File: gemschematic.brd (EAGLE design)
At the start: 90.2 x 61.9 mm, 57 parts, among them J1 USB, J3 QWIIC, J5 U.FL, Q1 2N3904, Q2 BSS138, Q3 MBT3904DW1T1, U1 ESP-WROOM-32NARROW, U2 AP2112K-3.3, U3 3.3V, U4 RFM96W, U5 CH340C, U6 BMP180, U7 STM32L073RZT6, X1 GPS_PA1010D

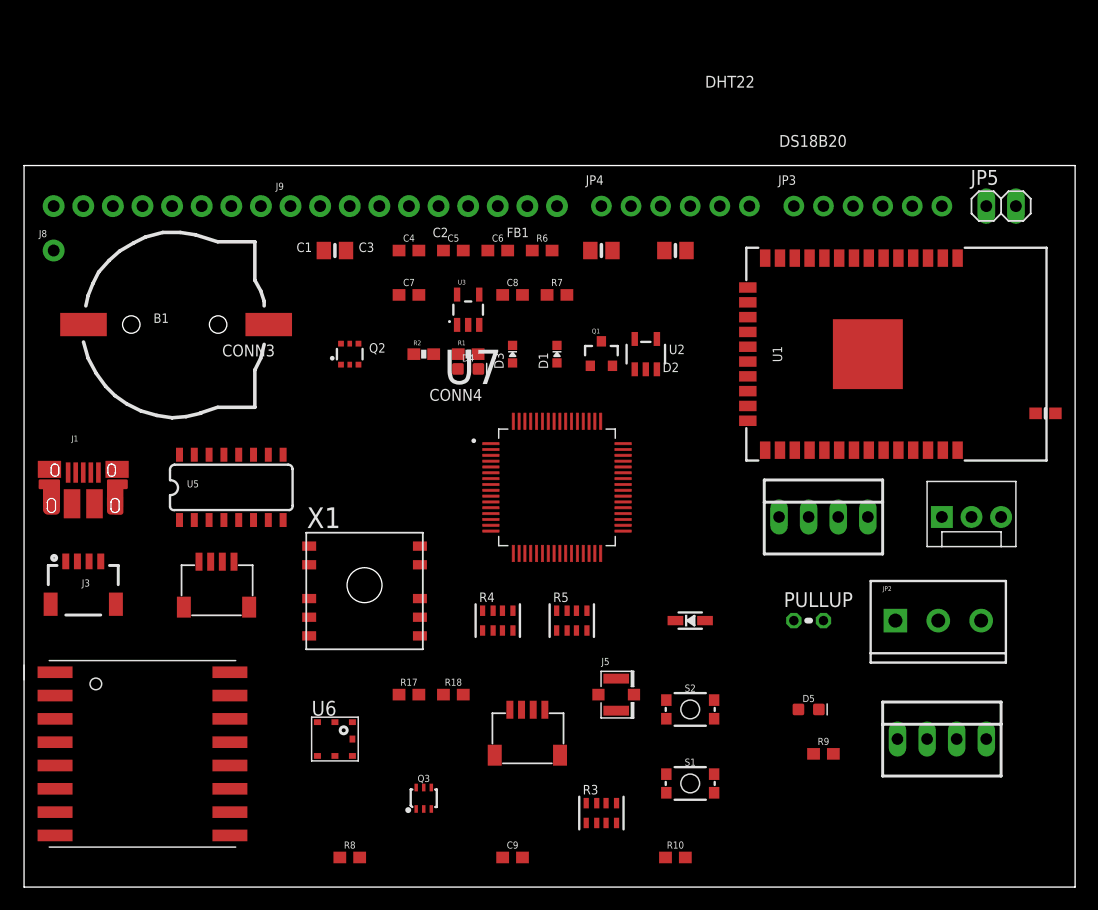
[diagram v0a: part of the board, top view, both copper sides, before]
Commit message: Add files via upload
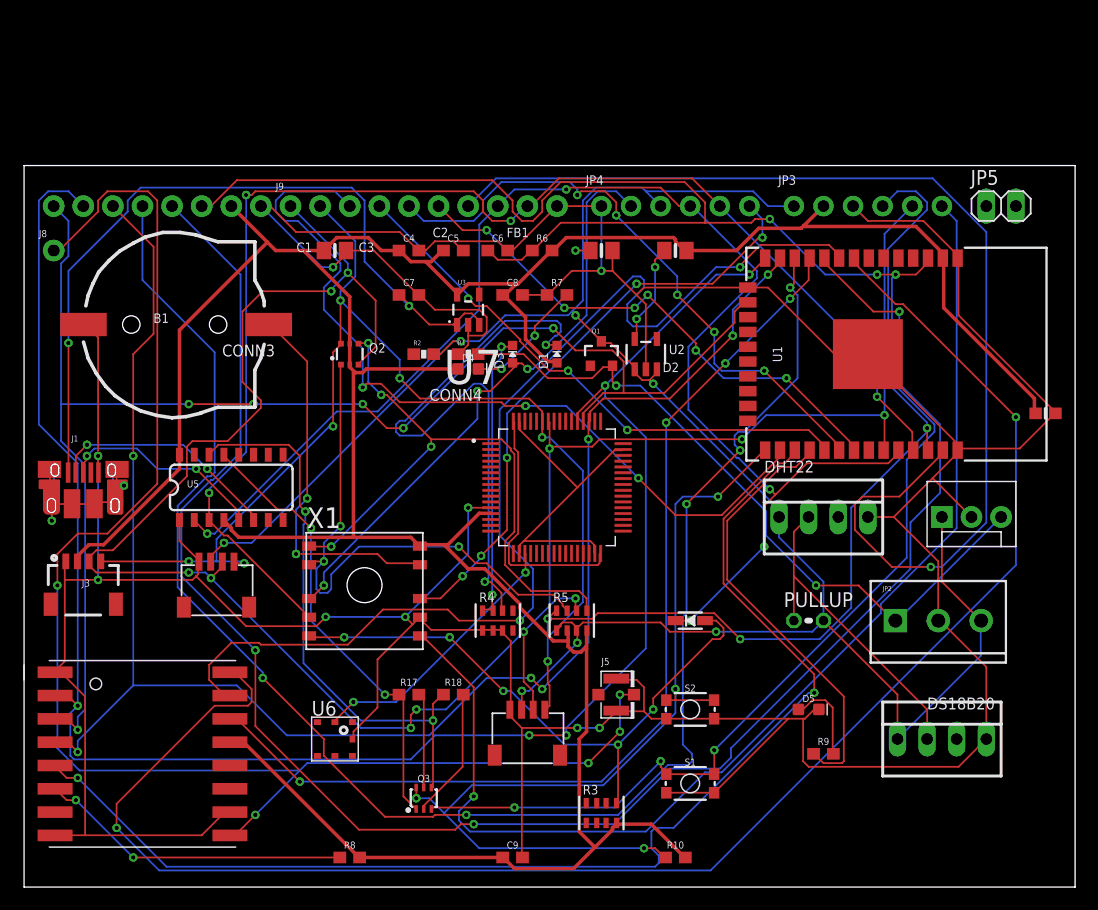
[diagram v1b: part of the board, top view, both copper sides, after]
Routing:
- net GND: track 0.00 -> 423.1 mm, vias 0 -> 9
- net 3.3V: track 0.00 -> 279.9 mm
- net SDA: track 0.00 -> 189.3 mm, vias 0 -> 11
- net VCC: track 0.00 -> 183.9 mm, vias 0 -> 8
- net SCL: track 0.00 -> 179.1 mm, vias 0 -> 10
- net RESET: track 0.00 -> 171.9 mm, vias 0 -> 6
- net MISO: track 0.00 -> 156.4 mm, vias 0 -> 5
- net IO25: track 0.00 -> 154.6 mm, vias 0 -> 3
- net RFM_DIO2/32: track 0.00 -> 142.8 mm, vias 0 -> 2
- net SCK: track 0.00 -> 141.3 mm, vias 0 -> 7
- net IO27: track 0.00 -> 140.8 mm, vias 0 -> 5
- net ANT: track 0.00 -> 127.0 mm, vias 0 -> 5
- net MOSI: track 0.00 -> 125.1 mm, vias 0 -> 6
- net RXI: track 0.00 -> 120.5 mm, vias 0 -> 5
- net TXO: track 0.00 -> 114.0 mm, vias 0 -> 4
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
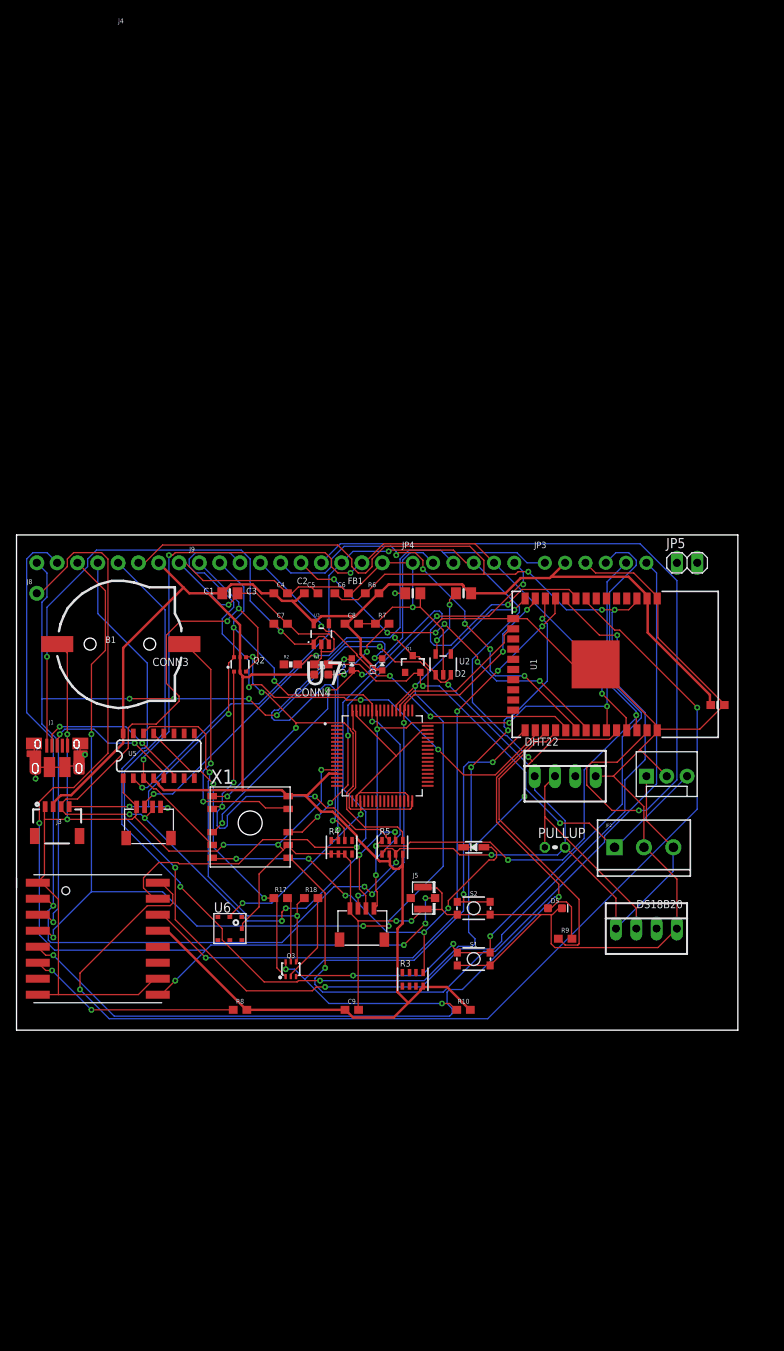
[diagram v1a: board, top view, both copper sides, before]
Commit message: Add files via upload
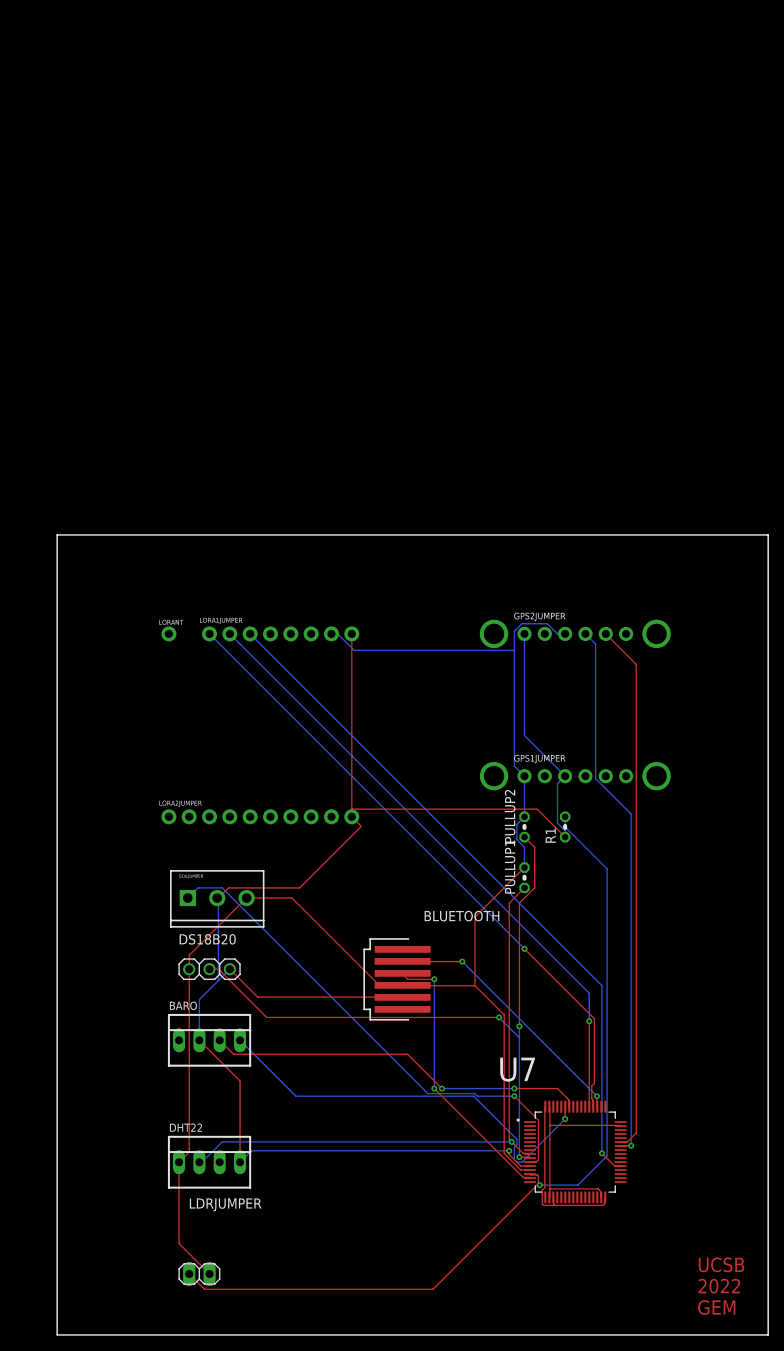
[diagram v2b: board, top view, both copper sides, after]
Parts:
- removed B1: (no value), microbuilder:CR1220-2
- removed C1: 0.1uF, microbuilder:0603-NO
- removed C2, C3: 10uF, microbuilder:0805-NO
- removed C4: 10uF, SparkFun-Capacitors:0603
- removed C5, C6: 0.1uF, SparkFun-Capacitors:0603
- removed C7, C8: 1.0uF, SparkFun-Capacitors:0603
- removed C9: 4.7uF, SparkFun-Capacitors:0603
- removed CONN3, CONN4: STEMMA_I2C_QT, microbuilder:JST_SH4
- removed D1: GREEN, microbuilder:CHIPLED_0603_NOOUTLINE
- removed D2: 1N4148, microbuilder:SOD-323
- removed D3: RED, microbuilder:CHIPLED_0603_NOOUTLINE
- removed D4: RED, SparkFun-LED:LED-0603
- removed D5: GREEN, SparkFun-LED:LED-0603
- removed FB1: FERRITE, microbuilder:0805-NO
- removed J1: USB, SparkFun-Connectors:USB-MICROB-PTH-MILL
- removed J3: QWIIC, SparkFun-Connectors:1X04_1MM_RA
- removed J4: (no value), SparkFun-Connectors:1X08_NO_SILK
- removed J5: U.FL, SparkFun-Connectors:U.FL
- removed J8: (no value), SparkFun-Connectors:1X01_NO_SILK
- removed J9: (no value), SparkFun-Connectors:1X10_NO_SILK
- removed JP1: DNP, SparkFun-Connectors:MOLEX-1X3
- removed JP2: (no value), SparkFun-Connectors:SCREWTERMINAL-3.5MM-3_LOCK.007S
- removed JP3, JP4: (no value), microbuilder:1X06_ROUND_70
- removed JP5: (no value), pinhead:1X02
- removed PULLUP: 10k, adafruit:0204V
- removed Q1: 2N3904, SparkFun-DiscreteSemi:SOT23-3
- removed Q2: BSS138, microbuilder:SOT363
- removed Q3: MBT3904DW1T1, esp32-thing-temp:SC70-6
- removed R10, R17, R18, R6, R8: 10k, SparkFun-Resistors:0603
- removed R2: 100, SparkFun-Resistors:0603-RES
- removed R3, R4, R5: 10K, microbuilder:RESPACK_4X0603
- removed R7, R9: 1k, SparkFun-Resistors:0603
- removed S1: RESET, SparkFun-Switches:TACTILE_SWITCH_SMD_4.6X2.8MM
- removed S2: 0, SparkFun-Switches:TACTILE_SWITCH_SMD_4.6X2.8MM
- removed U1: ESP-WROOM-32NARROW, esp32_lora_gateway:ESP-WROOM-32-NARROW
- removed U2: AP2112K-3.3, microbuilder:SOT23-5
- removed U3: 3.3V, SparkFun-IC-Power:SOT23-5
- removed U4: RFM96W, SparkX:RFM95/96/97/98W
- removed U5: CH340C, SparkFun-IC-Comms:SO016
- removed U6: BMP180, BMP180:BMP180
- removed X1: GPS_PA1010D, microbuilder:GPS_PA1010D
- added BARO: 22-23-2041, con-molex:22-23-2041
- added BLUETOOTH: 87438-06, con-molex:87438-06
- added GPS1JUMPER, GPS2JUMPER: (no value), microbuilder:1X06_ROUND_70
- added LDRJUMPER: (no value), pinhead:1X02
- added LORA1JUMPER: (no value), SparkFun-Connectors:1X08_NO_SILK
- added LORA2JUMPER: (no value), SparkFun-Connectors:1X10_NO_SILK
- added LORANT: (no value), SparkFun-Connectors:1X01_NO_SILK
- added PULLUP1, PULLUP2: 4.7k, adafruit:0204V
- added SOILJUMPER: (no value), SparkFun-Connectors:SCREWTERMINAL-3.5MM-3_LOCK.007S
- DS18B20: value 22-23-2041 -> (none); device con-molex:22-23-2041 -> adafruit:1X03
- R1: value 10k -> 270; device SparkFun-Resistors:0603-RES -> adafruit:0204V
- moved DHT22 65.6 mm to (19.1, 21.6)
- moved U7 55.1 mm to (64.8, 22.9)
- moved DS18B20 54.8 mm to (19.1, 45.7)
- moved R1 36.6 mm to (63.5, 63.5), turned to 90 degrees
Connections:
- removed net !DTR: Q3.1, R17.1, U5.13
- removed net !RTS: Q3.4, R18.1, U5.14
- removed net 0: Q3.6, R10.1, S2.3, S2.4, U1.25
- removed net D+: J1.D+, U5.5
- removed net D-: J1.D-, U5.6
- removed net DATA: DHT22.2, DS18B20.2, PULLUP.1
- removed net DHT22: U7.9
- removed net IO17: R9.1, U1.28
- removed net MISO: J4.2, U1.14, U4.MISO, U7.53
- removed net MOSI: J4.1, U1.16, U4.MOSI, U7.52
- removed net N$10: Q3.5, R17.2
- removed net N$12: Q3.2, R18.2
- removed net N$2: D1.C, R4.6
- removed net N$3: D3.C, R4.7, R4.8
- removed net N$4: D4.C, R7.2
- removed net N$5: D5.A, R9.2
- removed net OUT: FB1.1, U2.5
- removed net PC5: JP5.1
- removed net PF0: U6.6
- removed net PF1: U6.5
- removed net PHOTO: U7.8
- removed net PROBE1: Q1.1
- removed net PROBE2: R2.1
- removed net RFM_CS: U1.27, U4.NSS
- removed net RFM_DIO1/33: U1.9, U4.DIO1
- removed net RFM_DIO2/32: U1.8, U4.DIO2
- removed net RFM_INT/26: U1.11, U4.DIO0
- removed net RFM_RST: R8.1, U4.!RESET
- removed net RXI_3V: D2.A, R3.5, X1.5
- removed net SCK: J4.3, U1.13, U4.SCK, U7.51
- removed net SCL_3V: Q2.1, R5.7, X1.2
- removed net SDA_3V: Q2.4, R5.5, X1.1
- removed net SHIELD: J1.SHIELD, J1.SHIELD10, J1.SHIELD2, J1.SHIELD3, J1.SHIELD4, J1.SHIELD5, J1.SHIELD6, J1.SHIELD7, J1.SHIELD8, J1.SHIELD9
- removed net SIG: JP1.3, JP2.1, Q1.2, R1.2
- removed net SOIL: U7.11
- removed net TEMP: U7.10
- removed net USART_RX: U7.17
- removed net USART_TX: U7.16
- removed net VBACKUP: B1.+, X1.9
- removed net VDDIO: U6.3
- removed net V_USB: C7.1, J1.VBUS, U3.1, U3.3
- new net BTRX: BLUETOOTH.2, U7.51
- new net BTTX: BLUETOOTH.3, U7.15
- new net GPSRX: GPS2JUMPER.4, U7.42
- new net GPSTX: GPS2JUMPER.5, U7.43
- new net MISOLORA: LORA1JUMPER.2, U7.53
- new net MOSILORA: LORA1JUMPER.1, U7.52
- new net PA0LDR: LDRJUMPER.1, R1.2, U7.14
- new net PC1DHT: DHT22.2, PULLUP1.1, U7.9
- new net PC2DS18B20: DS18B20.2, PULLUP2.1, U7.10
- new net PC3SOIL: SOILJUMPER.1, U7.11
- new net SCKLORA: LORA1JUMPER.3, U7.37
- new net SCLBARO: BARO.3, U7.58
- new net SDABARO: BARO.4, U7.59
- new net VIN: BARO.1
- net !RESET: now also GPS1JUMPER.6; no longer JP3.6, X1.6
- net 1PPS: now also GPS2JUMPER.2; no longer D3.A, JP4.2, X1.3
- net 3.3V: now also GPS1JUMPER.2; no longer C1.1, C3.1, C4.1, C5.1, C8.1, C9.1, D1.A, D4.A, FB1.2, J3.2, J4.7, JP3.2, Q2.2, Q2.5, R10.2, R3.4, R5.2, R5.4, R6.2, R8.2, U1.2, U3.5, U4.3.3V, U5.16, U5.4, U7.13, X1.10
- net ANT: now also LORANT.1; no longer J5.FEED, J8.1, U4.ANT
- net GND: now also BARO.2, BLUETOOTH.5, DS18B20.3, GPS1JUMPER.3, GPS2JUMPER.1, LORA1JUMPER.8, LORA2JUMPER.10, SOILJUMPER.2; no longer B1.-, C1.2, C2.2, C3.2, C4.2, C5.2, C6.2, C7.2, C8.2, C9.2, CONN3.1, CONN4.1, D5.C, DS18B20.4, J1.GND, J3.1, J4.8, J5.1, J5.2, J9.10, JP1.2, JP2.2, JP3.3, JP4.1, R4.1, R4.2, R4.3, R7.1, S1.1, S1.2, S2.1, S2.2, U1.1, U1.15, U1.38, U1.GND, U2.2, U3.2, U4.GND@1, U4.GND@2, U4.GND@3, U5.1, U6.7, X1.7
- net IO18: now also LORA2JUMPER.5; no longer J9.5, U1.30
- net IO19: now also LORA2JUMPER.6; no longer J9.6, U1.31
- net IO23: now also LORA2JUMPER.7; no longer J9.7, U1.37
- net IO25: now also LORA1JUMPER.5; no longer J4.5, U1.10
- net IO27: now also LORA1JUMPER.4; no longer J4.4, U1.12
- net IO4: now also LORA2JUMPER.3; no longer J9.3, U1.26
- net IO5: now also LORA2JUMPER.4; no longer J9.4, U1.29
- net RESET: now also LORA1JUMPER.6; no longer C6.1, J4.6, Q3.3, R6.1, S1.3, S1.4, U1.3
- net RXI: now also LORA2JUMPER.8; no longer D2.C, J9.8, JP4.4, U1.34, U5.2
- net SCL: now also LORA2JUMPER.2; no longer CONN3.4, CONN4.4, J3.4, J9.2, JP3.4, Q2.6, R5.8, U1.36, U7.59
- net SDA: now also LORA2JUMPER.1; no longer CONN3.3, CONN4.3, J3.3, J9.1, JP3.5, Q2.3, R5.6, U1.33, U7.58
- net TXO: now also LORA2JUMPER.9; no longer J9.9, JP4.5, U1.35, U5.3, X1.4
- net VCC: now also BLUETOOTH.4, GPS1JUMPER.1, GPS2JUMPER.3, LDRJUMPER.2, LORA1JUMPER.7, PULLUP1.2, PULLUP2.2, SOILJUMPER.3, U7.13; no longer C2.1, CONN3.2, CONN4.2, JP1.1, JP2.3, JP3.1, JP4.3, PULLUP.2, Q1.3, R2.2, R5.1, R5.3, U2.1, U2.3
- net VDD: no longer U6.2
- net WAKEUP: now also GPS2JUMPER.6; no longer JP4.6, X1.8
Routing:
- net 3.3V: track 279.9 -> 0.00 mm
- net GND: track 423.1 -> 201.9 mm, vias 9 -> 1
- net SDA: track 189.3 -> 0.00 mm, vias 11 -> 0
- net SCL: track 179.1 -> 0.00 mm, vias 10 -> 0
- net RESET: track 171.9 -> 0.00 mm, vias 6 -> 0
- net MISO: track 156.4 -> 0.00 mm, vias 5 -> 0
- net IO25: track 154.6 -> 0.00 mm, vias 3 -> 0
- net RFM_DIO2/32: track 142.8 -> 0.00 mm, vias 2 -> 0
- net SCK: track 141.3 -> 0.00 mm, vias 7 -> 0
- net IO27: track 140.8 -> 0.00 mm, vias 5 -> 0
- net ANT: track 127.0 -> 0.00 mm, vias 5 -> 0
- net MOSI: track 125.1 -> 0.00 mm, vias 6 -> 0
- net RXI: track 120.5 -> 0.00 mm, vias 5 -> 0
- net TXO: track 114.0 -> 0.00 mm, vias 4 -> 0
- net PA0LDR: track 0.00 -> 106.7 mm, vias 0 -> 1
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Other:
- board size 90.2 x 61.9 mm -> 88.9 x 100 mm
- board text added: "UCSB 2022 GEM"
